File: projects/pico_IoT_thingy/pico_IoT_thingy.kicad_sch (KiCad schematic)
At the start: 58 parts, among them IC1 THVD1406DR, J1 Barrel_Jack_Switch, J2 QWIIC, J3 Conn_01x03, J4 Screw_Terminal_01x03, J5 Screw_Terminal_01x04, J6 Conn_02x05_Odd_Even, J7 Conn_01x02, K1 RT314A05, Q1 BC817, SW1 SW_SPST, SW2 SW_SPST, SW3 SW_DIP_x04, U1 TSR_1-2450, U2 SHT31-DIS, U3 TLV1117-33

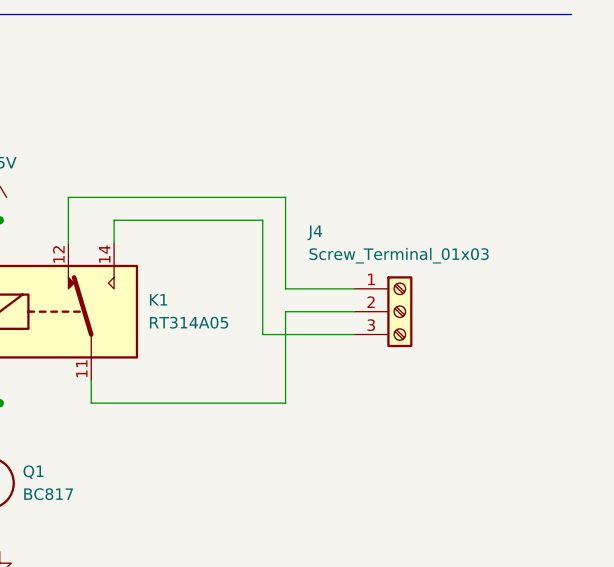
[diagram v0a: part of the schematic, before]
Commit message: Pico IoT thingy - logos and initial routing
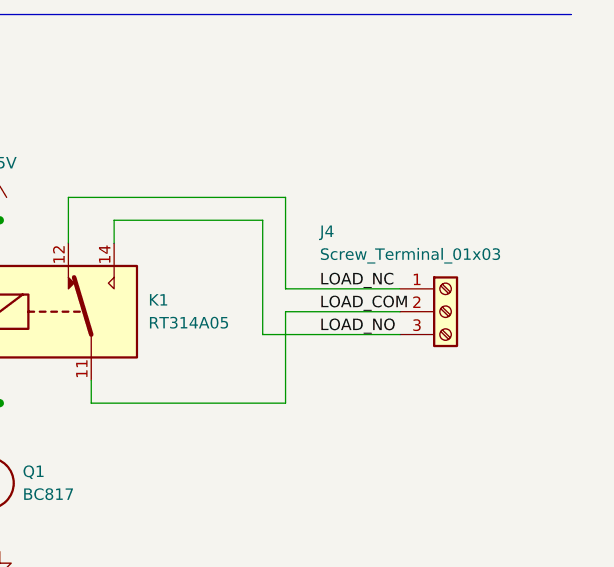
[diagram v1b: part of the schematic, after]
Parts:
- A1, D3, D5, D8, J2, J3, J4, J5: Mouser Ref (none) -> aliexpress
- C1, C3, C4, C5, C6, C7, C8, D2, D4, J1, J7, R1, R10, R11, R12, R13, R14, R15, R16, R17, R18, R19, R2, R20, R3, R4, R5, R6, R7, R8, R9, SW1, SW2: Mouser Ref (none) -> stash
- C2: Mouser Ref (none) -> 581-12065C225K4Z2A
- D1: Mouser Ref (none) -> 576-SMAJ24A
- D7: Mouser Ref (none) -> 576-SM712-02HTG
- F1: Mouser Ref (none) -> 652-MFSM100-2
- H1, H2, H3, H4, JP1: Mouser Ref (none) -> na
- IC1: Mouser Ref (none) -> 595-THVD1406DR
- J6: Mouser Ref (none) -> 200-MTSW10509GD490
- K1: Mouser Ref (none) -> 655-RT314A05
- Q1: Mouser Ref (none) -> 583-BC817
- SW3: Mouser Ref (none) -> 774-2194MST
- U1: Mouser Ref (none) -> 495-TSR1-2450E
- U2: Mouser Ref (none) -> 403-SHT31ADIS-B2.5KS
- U3: Mouser Ref (none) -> 595-TLV1117-33IDCYR
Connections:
- net LOAD_COM: now reaches J4.2 (Pin_2), K1.11
- net LOAD_NC: now reaches J4.1 (Pin_1), K1.12
- net LOAD_NO: now reaches J4.3 (Pin_3), K1.14
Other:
- moved on the sheet: J4
